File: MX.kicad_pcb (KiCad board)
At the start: 2 copper layers, 50.8 x 25.4 mm, 2 parts

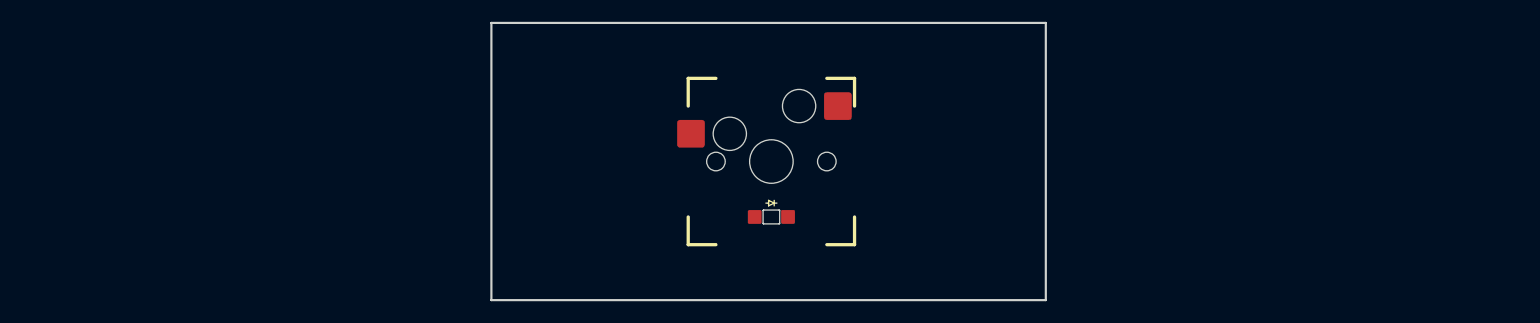
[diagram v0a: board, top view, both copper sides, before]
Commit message: Fixed names
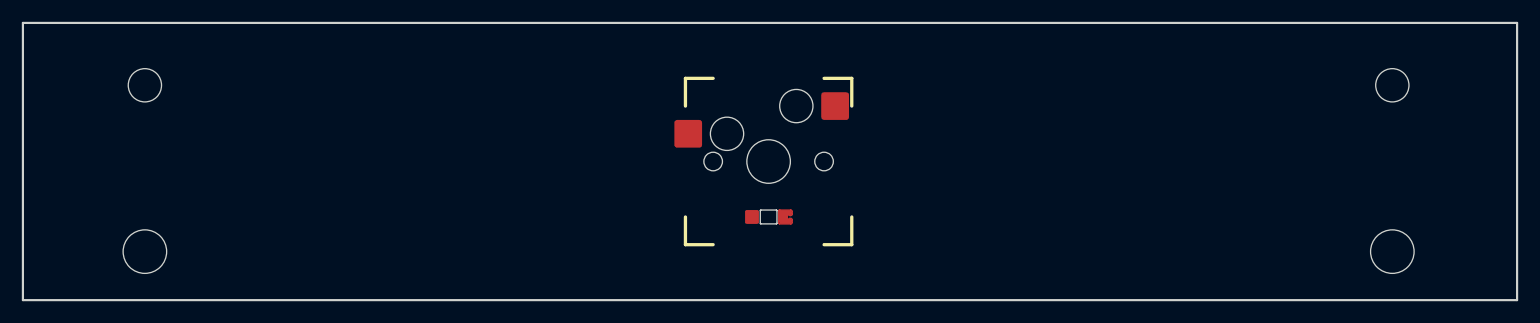
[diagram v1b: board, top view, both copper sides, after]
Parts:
- removed the SW** at (152.7, 88.9)
- added SW**: MX700H, Keyboard_switches:MX700H, F.Cu at (152.4, 88.9)
- moved LED** 0.25 mm to (152.4, 94.0)
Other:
- board size 50.8 x 25.4 mm -> 136.9 x 25.4 mm

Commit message: Upated MX700H and MX700HR
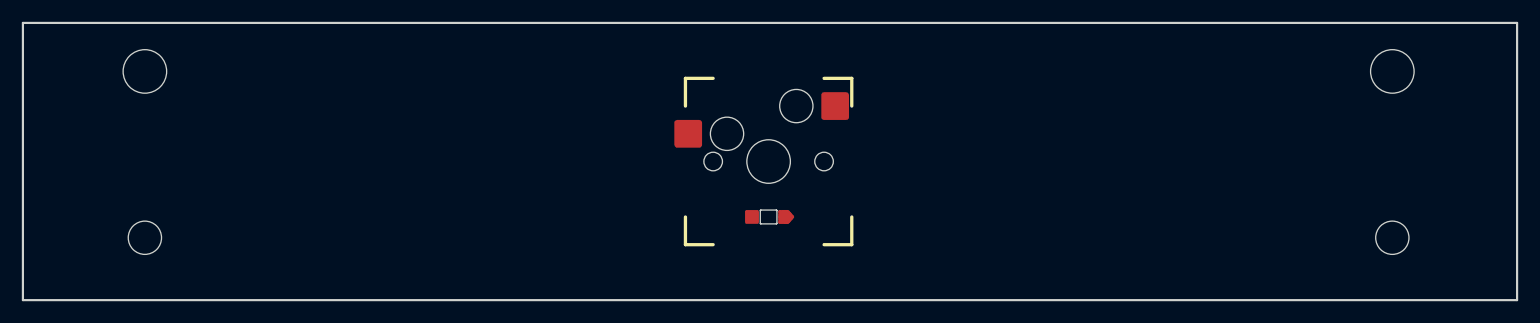
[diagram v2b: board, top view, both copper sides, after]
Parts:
- removed the SW** at (152.4, 88.9)
- added SW**: MX700HR, Keyboard_switches:MX700HR, F.Cu at (152.4, 88.9)
